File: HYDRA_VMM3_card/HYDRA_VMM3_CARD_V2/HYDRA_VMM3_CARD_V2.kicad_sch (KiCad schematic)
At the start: 22 parts, among them J1 ME1014010101011

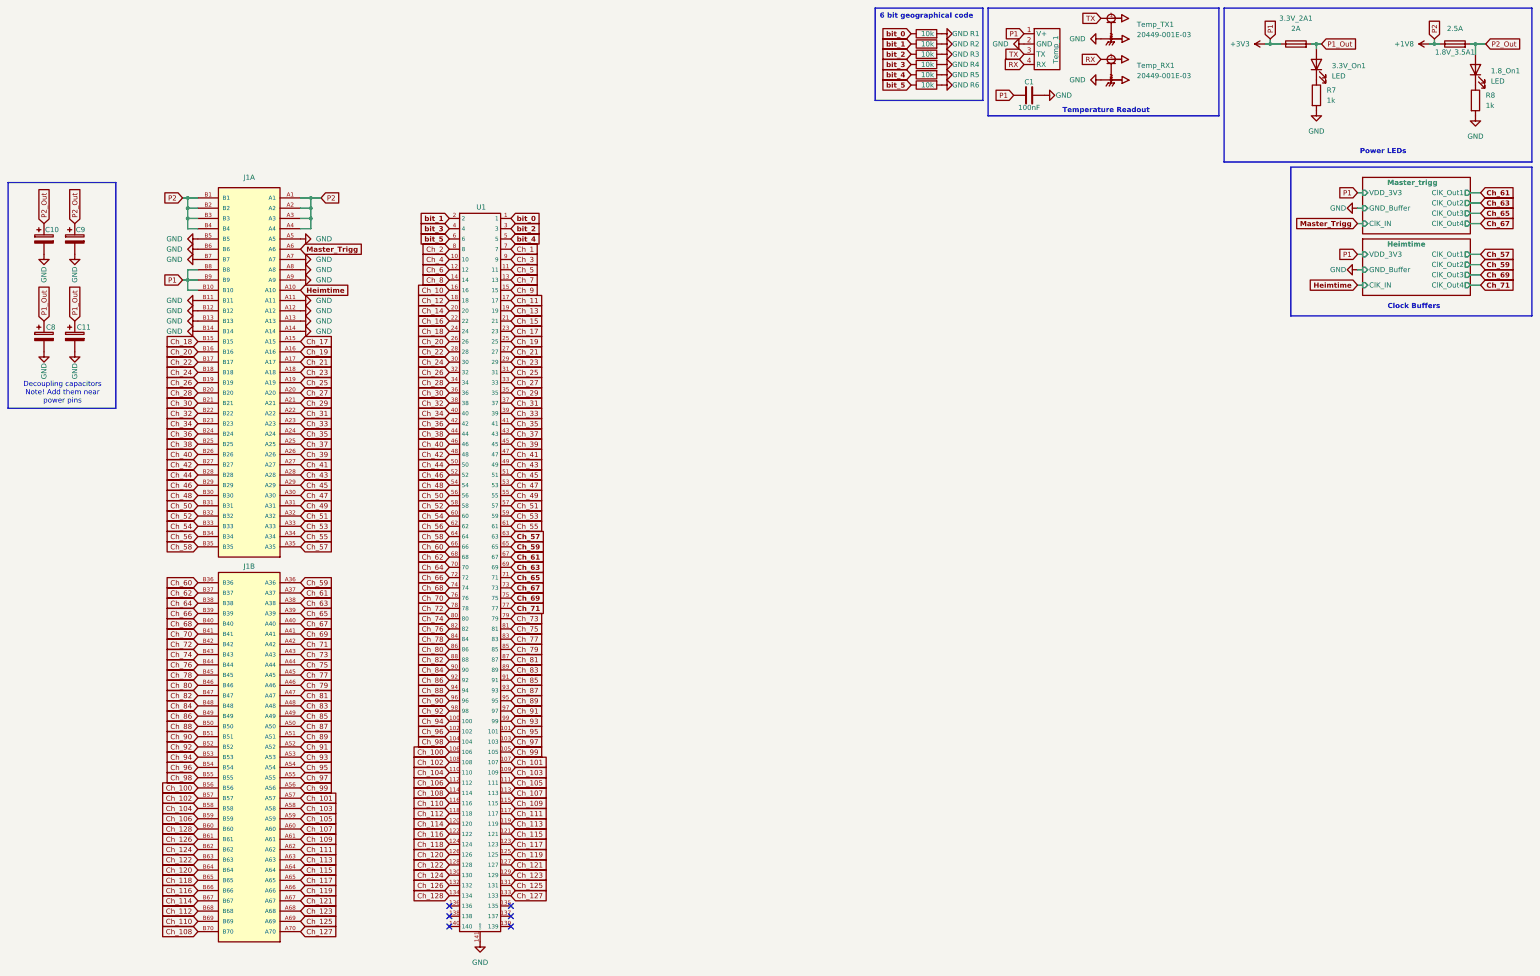
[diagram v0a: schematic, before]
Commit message: .
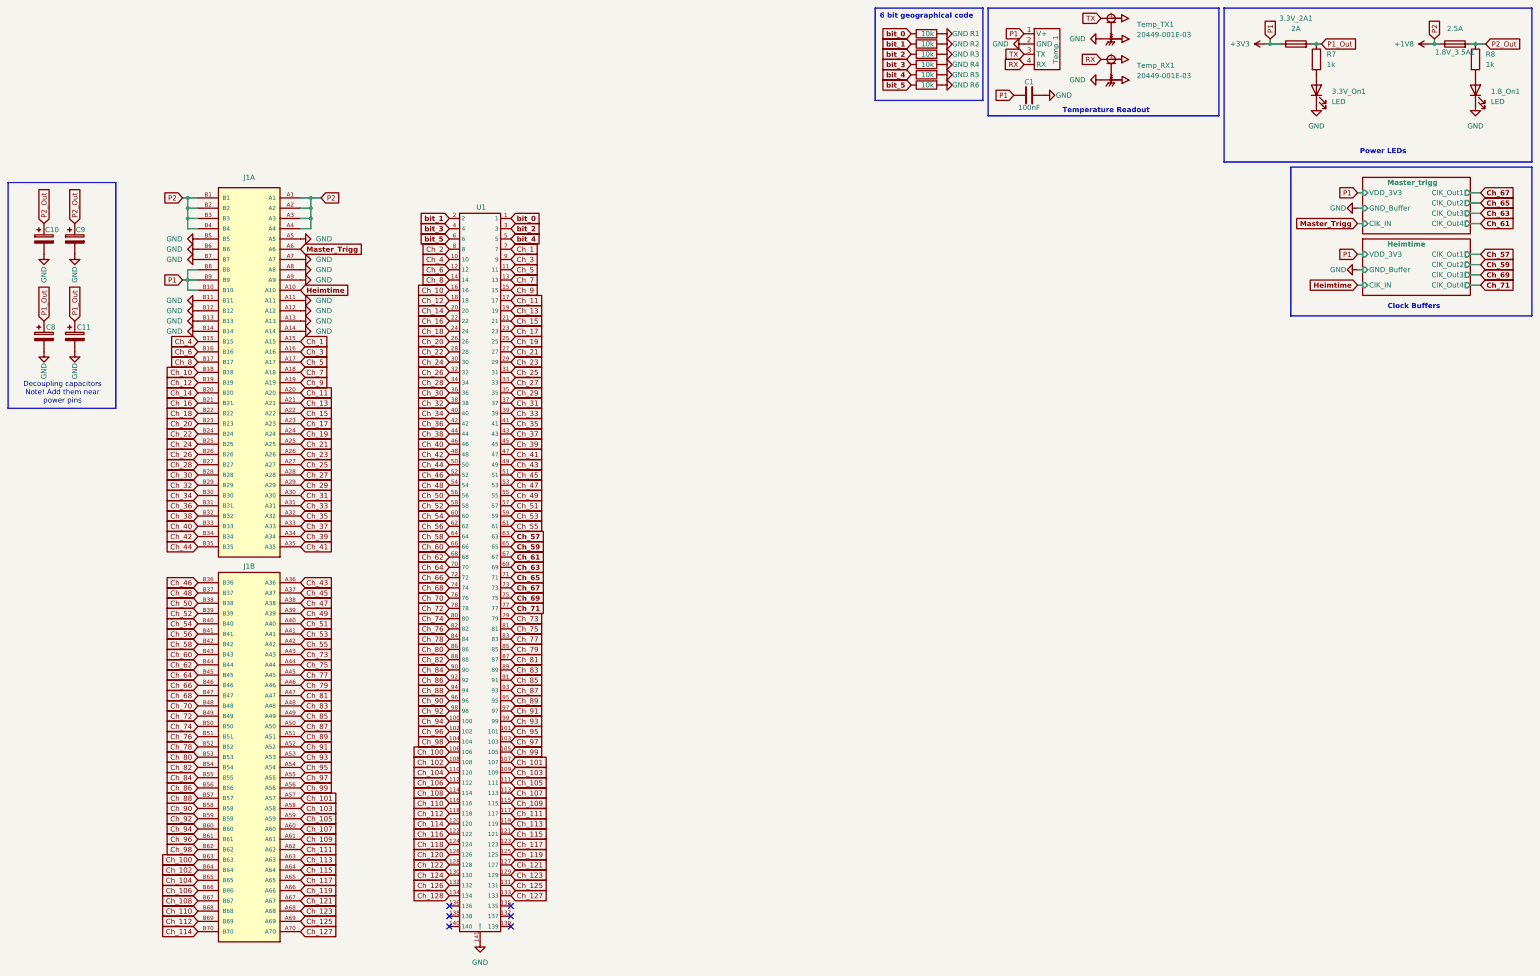
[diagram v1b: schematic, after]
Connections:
- net Ch_1: now also J1.A15
- net Ch_10: now also J1.B18
- net Ch_100: now also J1.B63; no longer J1.B56
- net Ch_102: now also J1.B64; no longer J1.B57
- net Ch_104: now also J1.B65; no longer J1.B58
- net Ch_106: now also J1.B66; no longer J1.B59
- net Ch_108: now also J1.B67; no longer J1.B70
- net Ch_11: now also J1.A20
- net Ch_110: now also J1.B68; no longer J1.B69
- net Ch_112: now also J1.B69; no longer J1.B68
- net Ch_114: now also J1.B70; no longer J1.B67
- net Ch_116: no longer J1.B66
- net Ch_118: no longer J1.B65
- net Ch_12: now also J1.B19
- net Ch_120: no longer J1.B64
- net Ch_122: no longer J1.B63
- net Ch_124: no longer J1.B62
- net Ch_126: no longer J1.B61
- net Ch_128: no longer J1.B60
- net Ch_13: now also J1.A21
- net Ch_14: now also J1.B20
- net Ch_15: now also J1.A22
- net Ch_16: now also J1.B21
- net Ch_17: now also J1.A23; no longer J1.A15
- net Ch_18: now also J1.B22; no longer J1.B15
- net Ch_19: now also J1.A24; no longer J1.A16
- net Ch_20: now also J1.B23; no longer J1.B16
- net Ch_21: now also J1.A25; no longer J1.A17
- net Ch_22: now also J1.B24; no longer J1.B17
- net Ch_23: now also J1.A26; no longer J1.A18
- net Ch_24: now also J1.B25; no longer J1.B18
- net Ch_25: now also J1.A27; no longer J1.A19
- net Ch_26: now also J1.B26; no longer J1.B19
- net Ch_27: now also J1.A28; no longer J1.A20
- net Ch_28: now also J1.B27; no longer J1.B20
- net Ch_29: now also J1.A29; no longer J1.A21
- net Ch_3: now also J1.A16
- net Ch_30: now also J1.B28; no longer J1.B21
- net Ch_31: now also J1.A30; no longer J1.A22
- net Ch_32: now also J1.B29; no longer J1.B22
- net Ch_33: now also J1.A31; no longer J1.A23
- net Ch_34: now also J1.B30; no longer J1.B23
- net Ch_35: now also J1.A32; no longer J1.A24
- net Ch_36: now also J1.B31; no longer J1.B24
- net Ch_37: now also J1.A33; no longer J1.A25
- net Ch_38: now also J1.B32; no longer J1.B25
- net Ch_39: now also J1.A34; no longer J1.A26
- net Ch_4: now also J1.B15
- net Ch_40: now also J1.B33; no longer J1.B26
- net Ch_41: now also J1.A35; no longer J1.A27
- net Ch_42: now also J1.B34; no longer J1.B27
- net Ch_43: now also J1.A36; no longer J1.A28
- net Ch_44: now also J1.B35; no longer J1.B28
- net Ch_45: now also J1.A37; no longer J1.A29
- net Ch_46: now also J1.B36; no longer J1.B29
- net Ch_47: now also J1.A38; no longer J1.A30
- net Ch_48: now also J1.B37; no longer J1.B30
- net Ch_49: now also J1.A39; no longer J1.A31
- net Ch_5: now also J1.A17
- net Ch_50: now also J1.B38; no longer J1.B31
- net Ch_51: now also J1.A40; no longer J1.A32
- net Ch_52: now also J1.B39; no longer J1.B32
- net Ch_53: now also J1.A41; no longer J1.A33
- net Ch_54: now also J1.B40; no longer J1.B33
- net Ch_55: now also J1.A42; no longer J1.A34
- net Ch_56: now also J1.B41; no longer J1.B34
- net Ch_57: no longer J1.A35
- net Ch_58: now also J1.B42; no longer J1.B35
- net Ch_59: no longer J1.A36
- net Ch_6: now also J1.B16
- net Ch_60: now also J1.B43; no longer J1.B36
- net Ch_61: no longer J1.A37
- net Ch_62: now also J1.B44; no longer J1.B37
- net Ch_63: no longer J1.A38
- net Ch_64: now also J1.B45; no longer J1.B38
- net Ch_65: no longer J1.A39
- net Ch_66: now also J1.B46; no longer J1.B39
- net Ch_67: no longer J1.A40
- net Ch_68: now also J1.B47; no longer J1.B40
- net Ch_69: no longer J1.A41
- net Ch_7: now also J1.A18
- net Ch_70: now also J1.B48; no longer J1.B41
- net Ch_71: no longer J1.A42
- net Ch_72: now also J1.B49; no longer J1.B42
- net Ch_74: now also J1.B50; no longer J1.B43
- net Ch_76: now also J1.B51; no longer J1.B44
- net Ch_78: now also J1.B52; no longer J1.B45
- net Ch_8: now also J1.B17
- net Ch_80: now also J1.B53; no longer J1.B46
- net Ch_82: now also J1.B54; no longer J1.B47
- net Ch_84: now also J1.B55; no longer J1.B48
- net Ch_86: now also J1.B56; no longer J1.B49
- net Ch_88: now also J1.B57; no longer J1.B50
- net Ch_9: now also J1.A19
- net Ch_90: now also J1.B58; no longer J1.B51
- net Ch_92: now also J1.B59; no longer J1.B52
- net Ch_94: now also J1.B60; no longer J1.B53
- net Ch_96: now also J1.B61; no longer J1.B54
- net Ch_98: now also J1.B62; no longer J1.B55
- net GND: now also 1.8_On1.1 (K), 3.3V_On1.1 (K); no longer R7.2, R8.2
- net P1_Out: now also R7.1; no longer 3.3V_On1.2 (A)
- net P2_Out: now also R8.1; no longer 1.8_On1.2 (A)
- new net: 1.8_On1.2 (A), R8.2
- new net: 3.3V_On1.2 (A), R7.2
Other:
- moved on the sheet: 1.8_On1, 3.3V_On1, R7, R8

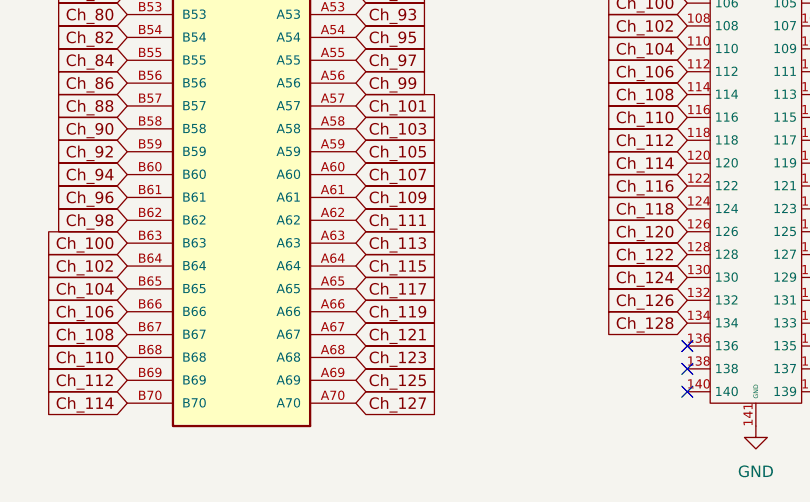
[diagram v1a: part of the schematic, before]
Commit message: .
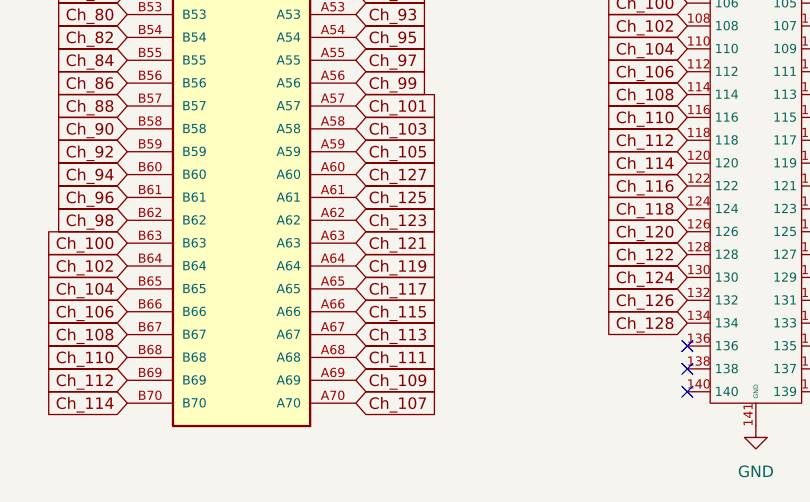
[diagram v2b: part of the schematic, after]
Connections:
- net Ch_107: now also J1.A70; no longer J1.A60
- net Ch_109: now also J1.A69; no longer J1.A61
- net Ch_111: now also J1.A68; no longer J1.A62
- net Ch_113: now also J1.A67; no longer J1.A63
- net Ch_115: now also J1.A66; no longer J1.A64
- net Ch_119: now also J1.A64; no longer J1.A66
- net Ch_121: now also J1.A63; no longer J1.A67
- net Ch_123: now also J1.A62; no longer J1.A68
- net Ch_125: now also J1.A61; no longer J1.A69
- net Ch_127: now also J1.A60; no longer J1.A70
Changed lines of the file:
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@@
 	(global_label "Ch_111"
 		(shape input)
-		(at 101.6 222.25 0)
+		(at 101.6 237.49 0)
 		(fields_autoplaced yes)
 		(effects
@@
 		)
 		(property "Intersheetrefs" "${INTERSHEET_REFS}"
-			(at 111.6003 222.25 0)
+			(at 111.6003 237.49 0)
 			(effects
 				(font
@@
 	(global_label "Ch_113"
 		(shape input)
-		(at 101.6 224.79 0)
+		(at 101.6 234.95 0)
 		(fields_autoplaced yes)
 		(effects
@@
 		)
 		(property "Intersheetrefs" "${INTERSHEET_REFS}"
-			(at 111.6003 224.79 0)
+			(at 111.6003 234.95 0)
 			(effects
 				(font
@@
 	(global_label "Ch_107"
 		(shape input)
-		(at 101.6 217.17 0)
+		(at 101.6 242.57 0)
 		(fields_autoplaced yes)
 		(effects
@@
 		)
 		(property "Intersheetrefs" "${INTERSHEET_REFS}"
-			(at 111.6003 217.17 0)
+			(at 111.6003 242.57 0)
 			(effects
 				(font
@@
 	(global_label "Ch_125"
 		(shape input)
-		(at 101.6 240.03 0)
+		(at 101.6 219.71 0)
 		(fields_autoplaced yes)
 		(effects
@@
 		)
 		(property "Intersheetrefs" "${INTERSHEET_REFS}"
-			(at 111.6003 240.03 0)
+			(at 111.6003 219.71 0)
 			(effects
 				(font
@@
 	(global_label "Ch_115"
 		(shape input)
-		(at 101.6 227.33 0)
+		(at 101.6 232.41 0)
 		(fields_autoplaced yes)
 		(effects
@@
 		)
 		(property "Intersheetrefs" "${INTERSHEET_REFS}"
-			(at 111.6003 227.33 0)
+			(at 111.6003 232.41 0)
 			(effects
 				(font
@@
 	(global_label "Ch_121"
 		(shape input)
-		(at 101.6 234.95 0)
+		(at 101.6 224.79 0)
 		(fields_autoplaced yes)
 		(effects
@@
 		)
 		(property "Intersheetrefs" "${INTERSHEET_REFS}"
-			(at 111.6003 234.95 0)
+			(at 111.6003 224.79 0)
 			(effects
 				(font
@@
 	(global_label "Ch_109"
 		(shape input)
-		(at 101.6 219.71 0)
+		(at 101.6 240.03 0)
 		(fields_autoplaced yes)
 		(effects
@@
 		)
 		(property "Intersheetrefs" "${INTERSHEET_REFS}"
-			(at 111.6003 219.71 0)
+			(at 111.6003 240.03 0)
 			(effects
 				(font
@@
 	(global_label "Ch_127"
 		(shape input)
-		(at 101.6 242.57 0)
+		(at 101.6 217.17 0)
 		(fields_autoplaced yes)
 		(effects
@@
 		)
 		(property "Intersheetrefs" "${INTERSHEET_REFS}"
-			(at 111.6003 242.57 0)
+			(at 111.6003 217.17 0)
 			(effects
 				(font
@@
 	(global_label "Ch_123"
 		(shape input)
-		(at 101.6 237.49 0)
+		(at 101.6 222.25 0)
 		(fields_autoplaced yes)
 		(effects
@@
 		)
 		(property "Intersheetrefs" "${INTERSHEET_REFS}"
-			(at 111.6003 237.49 0)
+			(at 111.6003 222.25 0)
 			(effects
 				(font
@@
 	(global_label "Ch_119"
 		(shape input)
-		(at 101.6 232.41 0)
+		(at 101.6 227.33 0)
 		(fields_autoplaced yes)
 		(effects
@@
 		)
 		(property "Intersheetrefs" "${INTERSHEET_REFS}"
-			(at 111.6003 232.41 0)
+			(at 111.6003 227.33 0)
 			(effects
 				(font

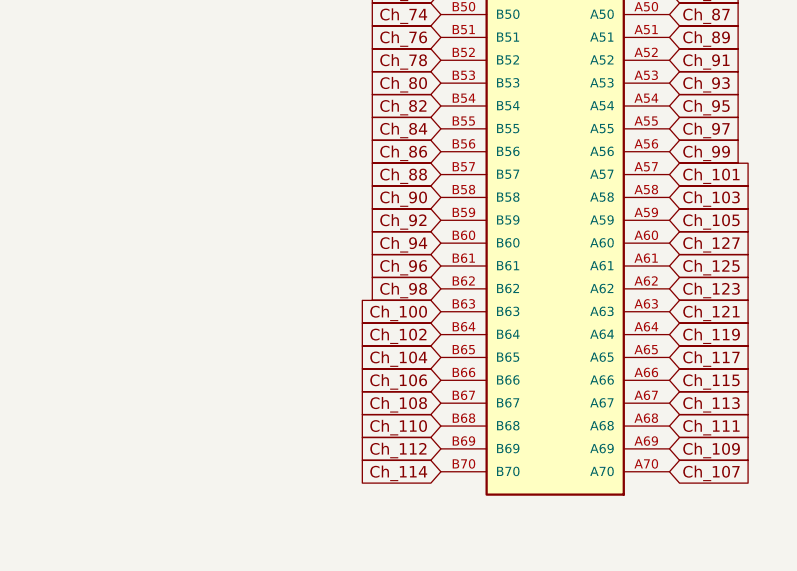
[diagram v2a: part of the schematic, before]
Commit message: .
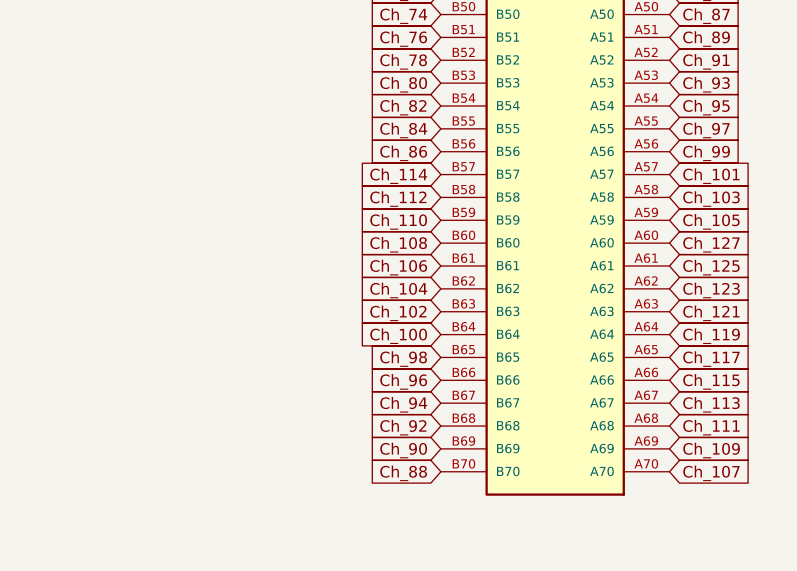
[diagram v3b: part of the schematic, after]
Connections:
- net Ch_100: now also J1.B64; no longer J1.B63
- net Ch_102: now also J1.B63; no longer J1.B64
- net Ch_104: now also J1.B62; no longer J1.B65
- net Ch_106: now also J1.B61; no longer J1.B66
- net Ch_108: now also J1.B60; no longer J1.B67
- net Ch_110: now also J1.B59; no longer J1.B68
- net Ch_112: now also J1.B58; no longer J1.B69
- net Ch_114: now also J1.B57; no longer J1.B70
- net Ch_88: now also J1.B70; no longer J1.B57
- net Ch_90: now also J1.B69; no longer J1.B58
- net Ch_92: now also J1.B68; no longer J1.B59
- net Ch_94: now also J1.B67; no longer J1.B60
- net Ch_96: now also J1.B66; no longer J1.B61
- net Ch_98: now also J1.B65; no longer J1.B62
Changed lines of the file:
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@@
 	(global_label "Ch_104"
 		(shape input)
-		(at 76.2 229.87 180)
+		(at 76.2 222.25 180)
 		(fields_autoplaced yes)
 		(effects
@@
 		)
 		(property "Intersheetrefs" "${INTERSHEET_REFS}"
-			(at 66.1997 229.87 0)
+			(at 66.1997 222.25 0)
 			(effects
 				(font
@@
 	(global_label "Ch_108"
 		(shape input)
-		(at 76.2 234.95 180)
+		(at 76.2 217.17 180)
 		(fields_autoplaced yes)
 		(effects
@@
 		)
 		(property "Intersheetrefs" "${INTERSHEET_REFS}"
-			(at 66.1997 234.95 0)
+			(at 66.1997 217.17 0)
 			(effects
 				(font
@@
 	(global_label "Ch_98"
 		(shape input)
-		(at 76.2 222.25 180)
+		(at 76.2 229.87 180)
 		(fields_autoplaced yes)
 		(effects
@@
 		)
 		(property "Intersheetrefs" "${INTERSHEET_REFS}"
-			(at 67.4092 222.25 0)
+			(at 67.4092 229.87 0)
 			(effects
 				(font
@@
 	(global_label "Ch_110"
 		(shape input)
-		(at 76.2 237.49 180)
+		(at 76.2 214.63 180)
 		(fields_autoplaced yes)
 		(effects
@@
 		)
 		(property "Intersheetrefs" "${INTERSHEET_REFS}"
-			(at 66.1997 237.49 0)
+			(at 66.1997 214.63 0)
 			(effects
 				(font
@@
 	(global_label "Ch_100"
 		(shape input)
-		(at 76.2 224.79 180)
+		(at 76.2 227.33 180)
 		(fields_autoplaced yes)
 		(effects
@@
 		)
 		(property "Intersheetrefs" "${INTERSHEET_REFS}"
-			(at 66.1997 224.79 0)
+			(at 66.1997 227.33 0)
 			(effects
 				(font
@@
 	(global_label "Ch_88"
 		(shape input)
-		(at 76.2 209.55 180)
+		(at 76.2 242.57 180)
 		(fields_autoplaced yes)
 		(effects
@@
 		)
 		(property "Intersheetrefs" "${INTERSHEET_REFS}"
-			(at 67.4092 209.55 0)
+			(at 67.4092 242.57 0)
 			(effects
 				(font
@@
 	(global_label "Ch_114"
 		(shape input)
-		(at 76.2 242.57 180)
+		(at 76.2 209.55 180)
 		(fields_autoplaced yes)
 		(effects
@@
 		)
 		(property "Intersheetrefs" "${INTERSHEET_REFS}"
-			(at 66.1997 242.57 0)
+			(at 66.1997 209.55 0)
 			(effects
 				(font
@@
 	(global_label "Ch_94"
 		(shape input)
-		(at 76.2 217.17 180)
+		(at 76.2 234.95 180)
 		(fields_autoplaced yes)
 		(effects
@@
 		)
 		(property "Intersheetrefs" "${INTERSHEET_REFS}"
-			(at 67.4092 217.17 0)
+			(at 67.4092 234.95 0)
 			(effects
 				(font
@@
 	(global_label "Ch_92"
 		(shape input)
-		(at 76.2 214.63 180)
+		(at 76.2 237.49 180)
 		(fields_autoplaced yes)
 		(effects
@@
 		)
 		(property "Intersheetrefs" "${INTERSHEET_REFS}"
-			(at 67.4092 214.63 0)
+			(at 67.4092 237.49 0)
 			(effects
 				(font
@@
 	(global_label "Ch_90"
 		(shape input)
-		(at 76.2 212.09 180)
+		(at 76.2 240.03 180)
 		(fields_autoplaced yes)
 		(effects
@@
 		)
 		(property "Intersheetrefs" "${INTERSHEET_REFS}"
-			(at 67.4092 212.09 0)
+			(at 67.4092 240.03 0)
 			(effects
 				(font
@@
 	(global_label "Ch_102"
 		(shape input)
-		(at 76.2 227.33 180)
+		(at 76.2 224.79 180)
 		(fields_autoplaced yes)
 		(effects
@@
 		)
 		(property "Intersheetrefs" "${INTERSHEET_REFS}"
-			(at 66.1997 227.33 0)
+			(at 66.1997 224.79 0)
 			(effects
 				(font
@@
 	(global_label "Ch_112"
 		(shape input)
-		(at 76.2 240.03 180)
+		(at 76.2 212.09 180)
 		(fields_autoplaced yes)
 		(effects
@@
 		)
 		(property "Intersheetrefs" "${INTERSHEET_REFS}"
-			(at 66.1997 240.03 0)
+			(at 66.1997 212.09 0)
 			(effects
 				(font
@@
 	(global_label "Ch_96"
 		(shape input)
-		(at 76.2 219.71 180)
+		(at 76.2 232.41 180)
 		(fields_autoplaced yes)
 		(effects
@@
 		)
 		(property "Intersheetrefs" "${INTERSHEET_REFS}"
-			(at 67.4092 219.71 0)
+			(at 67.4092 232.41 0)
 			(effects
 				(font
@@
 	(global_label "Ch_106"
 		(shape input)
-		(at 76.2 232.41 180)
+		(at 76.2 219.71 180)
 		(fields_autoplaced yes)
 		(effects
@@
 		)
 		(property "Intersheetrefs" "${INTERSHEET_REFS}"
-			(at 66.1997 232.41 0)
+			(at 66.1997 219.71 0)
 			(effects
 				(font
